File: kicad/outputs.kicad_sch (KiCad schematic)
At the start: 50 parts, among them J4 OUT Q1, J5 OUT Q2, J6 OUT Q3, J7 OUT Q4, J8 OUT Q5, J9 OUT Q6, Q1 AOD4184A, Q2 AOD4184A, Q3 AOD4184A, Q4 AOD4184A, Q5 AOD4184A, Q6 AOD4184A, U3 74HCT244D

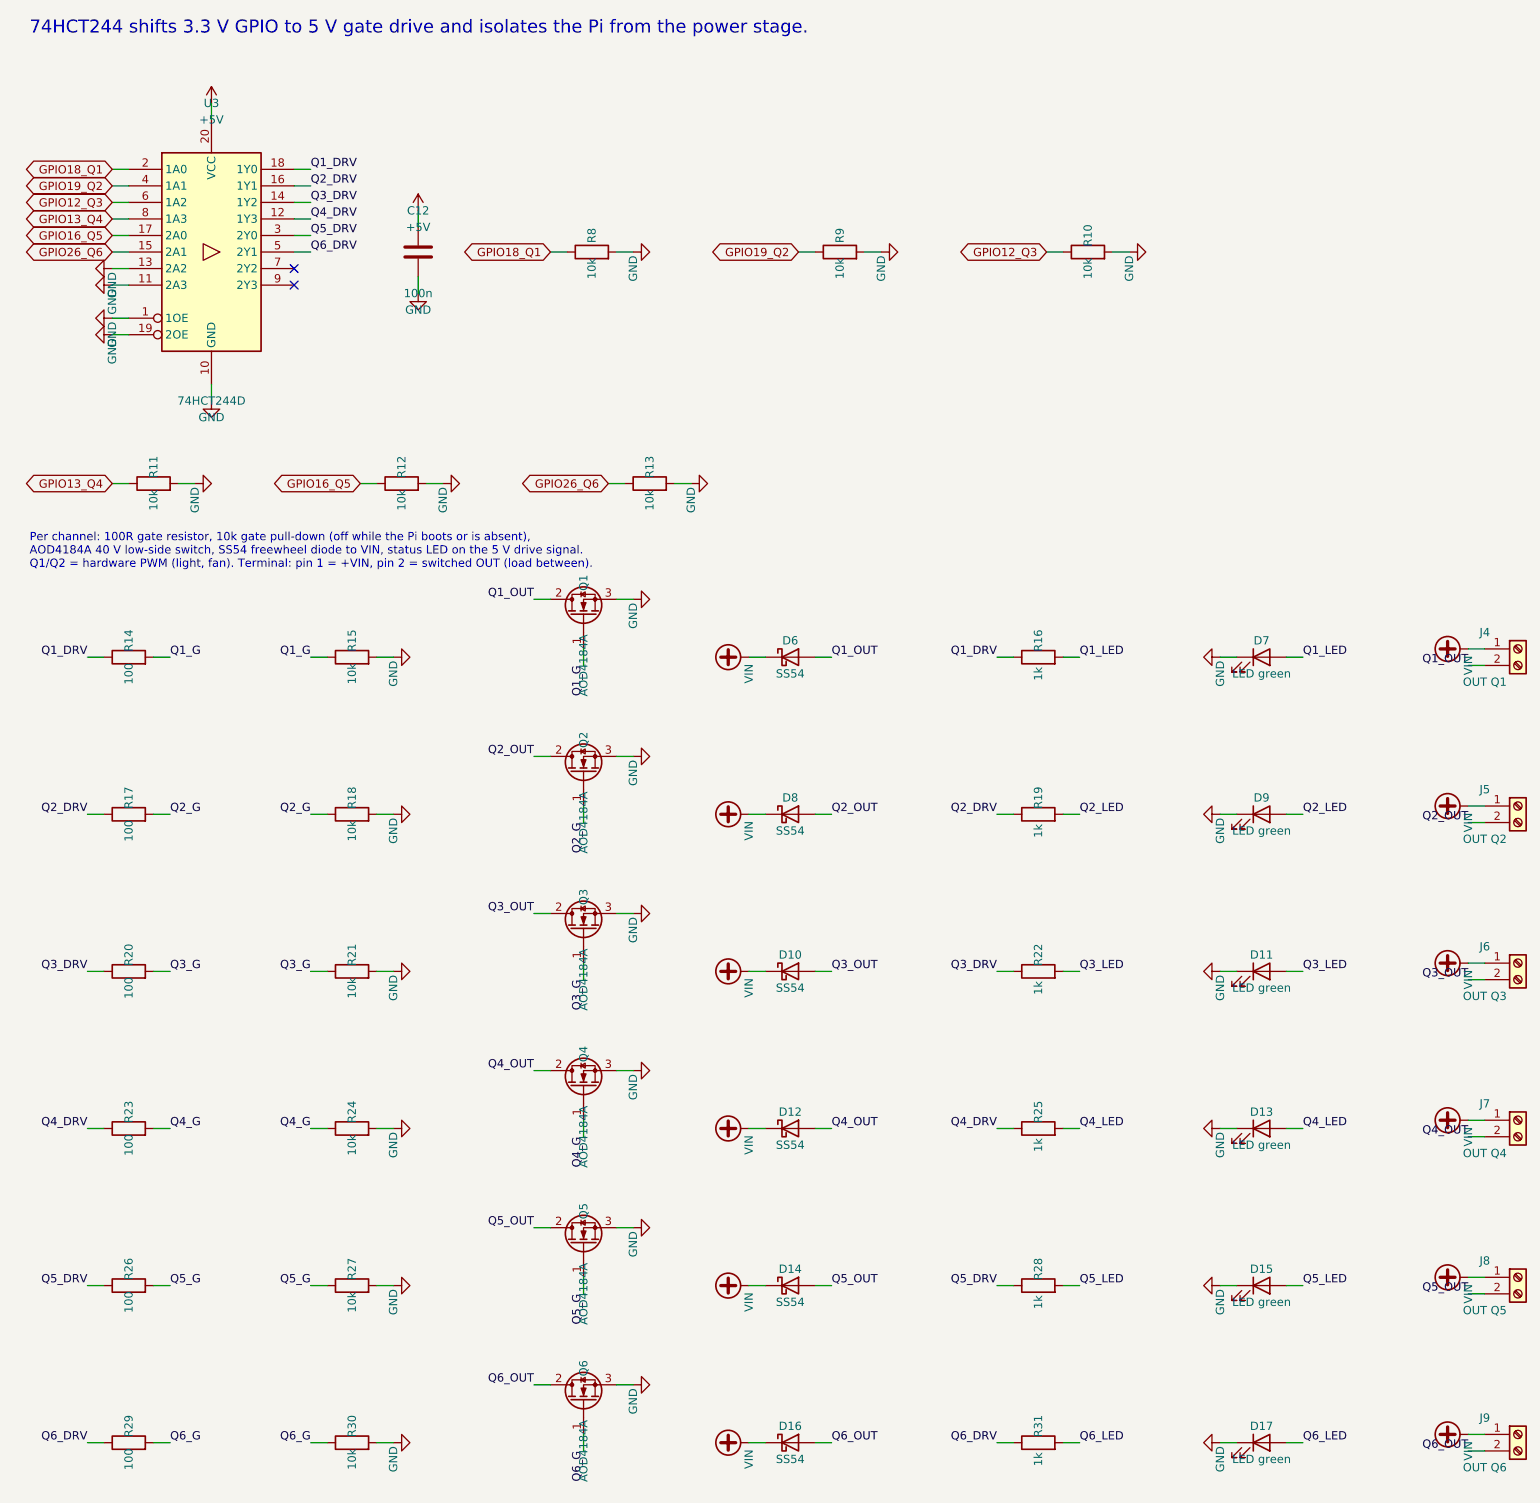
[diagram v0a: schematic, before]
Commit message: kicad: routing progress (by hand)
Co-Authored-By: Claude Opus 5.5 (1M context) <noreply@anthropic.com>
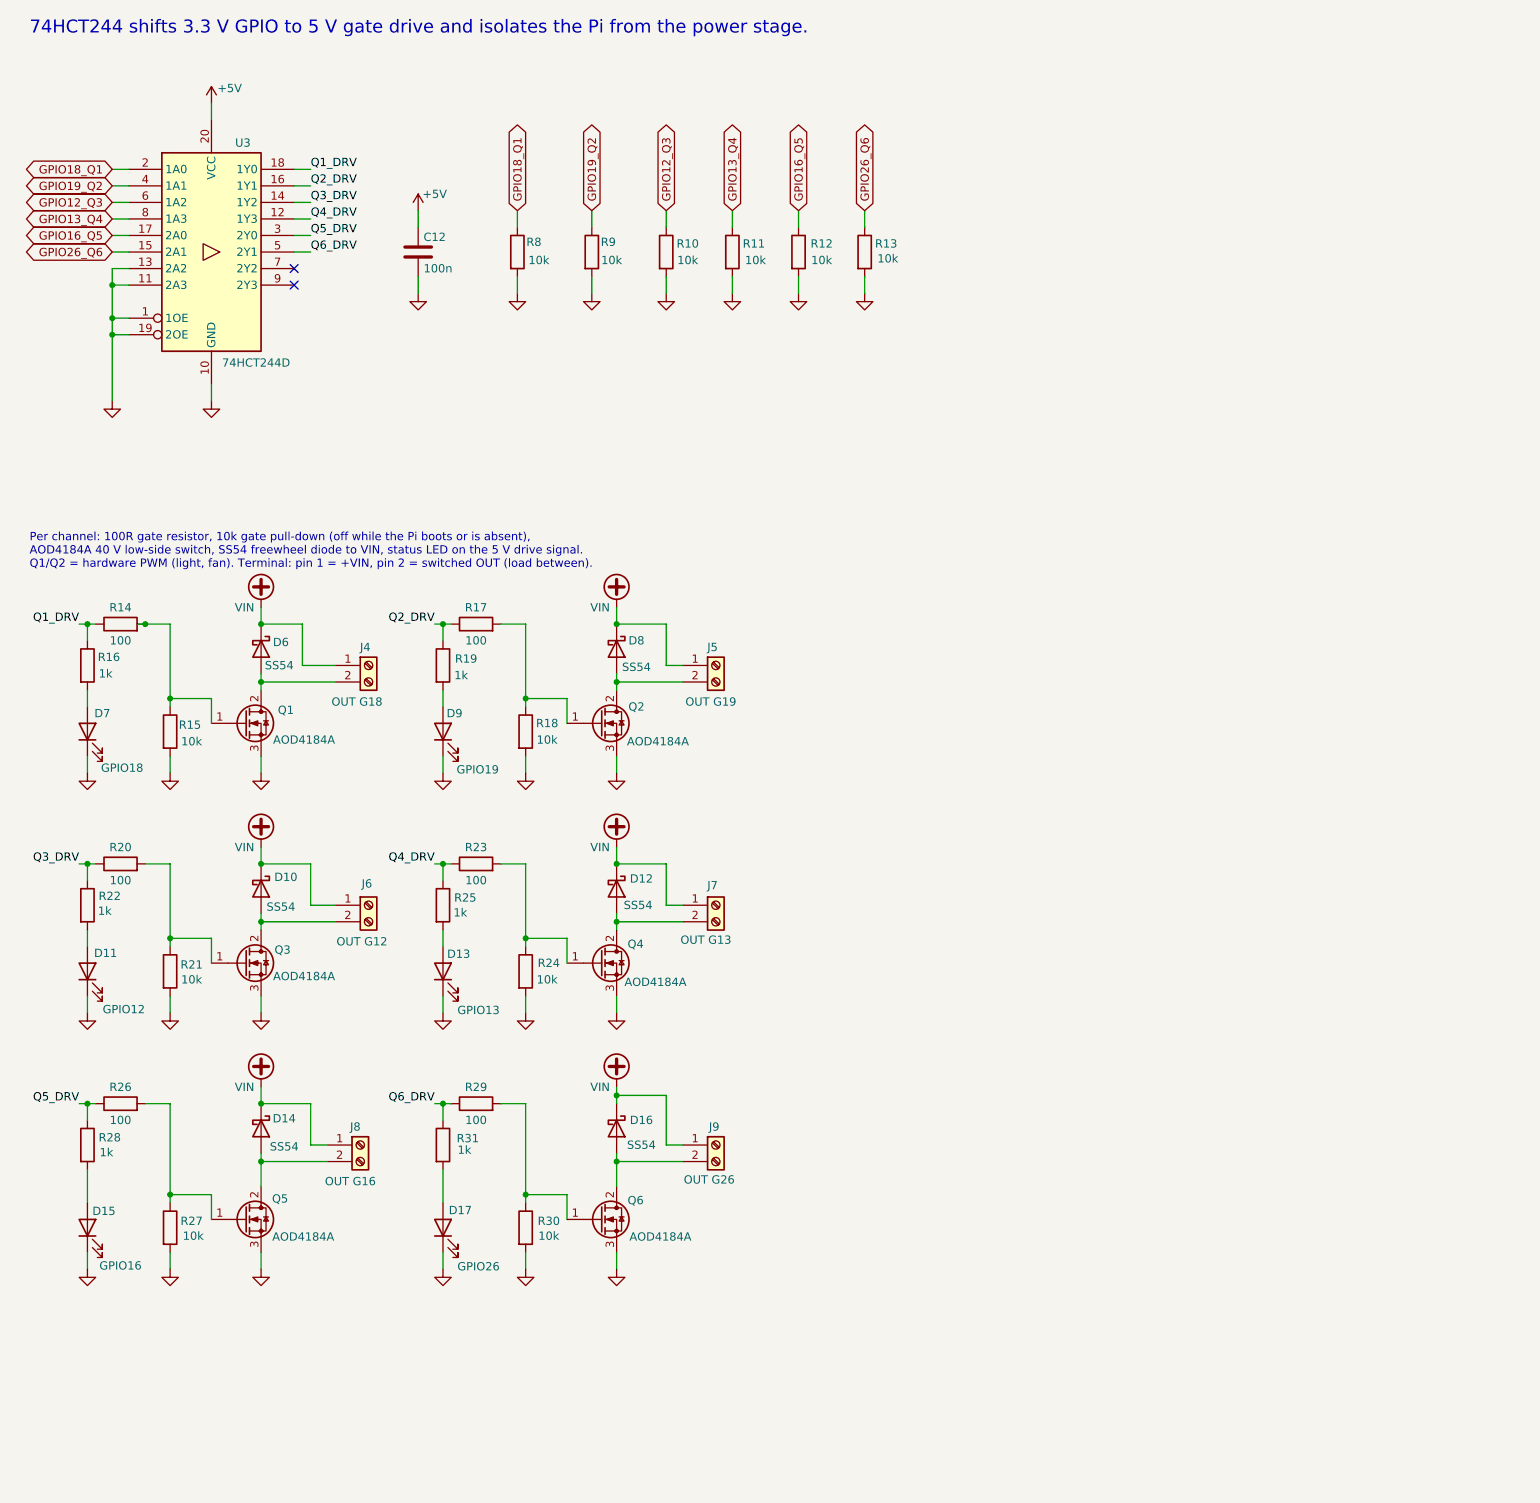
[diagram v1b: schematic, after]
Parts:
- D11: value LED green -> GPIO12
- D13: value LED green -> GPIO13
- D15: value LED green -> GPIO16
- D17: value LED green -> GPIO26
- D7: value LED green -> GPIO18
- D9: value LED green -> GPIO19
- J4: value OUT Q1 -> OUT G18
- J5: value OUT Q2 -> OUT G19
- J6: value OUT Q3 -> OUT G12
- J7: value OUT Q4 -> OUT G13
- J8: value OUT Q5 -> OUT G16
- J9: value OUT Q6 -> OUT G26
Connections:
- net Q1_G: no longer names the net of Q1.1 (G), R14.2, R15.1
- net Q1_LED: no longer names the net of D7.2 (A), R16.2
- net Q1_OUT: no longer names the net of D6.2 (A), J4.2 (Pin_2), Q1.2 (D)
- net Q2_G: no longer names the net of Q2.1 (G), R17.2, R18.1
- net Q2_LED: no longer names the net of D9.2 (A), R19.2
- net Q2_OUT: no longer names the net of D8.2 (A), J5.2 (Pin_2), Q2.2 (D)
- net Q3_G: no longer names the net of Q3.1 (G), R20.2, R21.1
- net Q3_LED: no longer names the net of D11.2 (A), R22.2
- net Q3_OUT: no longer names the net of D10.2 (A), J6.2 (Pin_2), Q3.2 (D)
- net Q4_G: no longer names the net of Q4.1 (G), R23.2, R24.1
- net Q4_LED: no longer names the net of D13.2 (A), R25.2
- net Q4_OUT: no longer names the net of D12.2 (A), J7.2 (Pin_2), Q4.2 (D)
- net Q5_G: no longer names the net of Q5.1 (G), R26.2, R27.1
- net Q5_LED: no longer names the net of D15.2 (A), R28.2
- net Q5_OUT: no longer names the net of D14.2 (A), J8.2 (Pin_2), Q5.2 (D)
- net Q6_G: no longer names the net of Q6.1 (G), R29.2, R30.1
- net Q6_LED: no longer names the net of D17.2 (A), R31.2
- net Q6_OUT: no longer names the net of D16.2 (A), J9.2 (Pin_2), Q6.2 (D)
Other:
- moved on the sheet: D10, D11, D12, D13, D14, D15, D16, D17, D6, D7, D8, D9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
